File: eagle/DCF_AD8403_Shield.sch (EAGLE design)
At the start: 21 parts, among them IC1 TL072P, IC2 AD8403-100, J1 DCIN

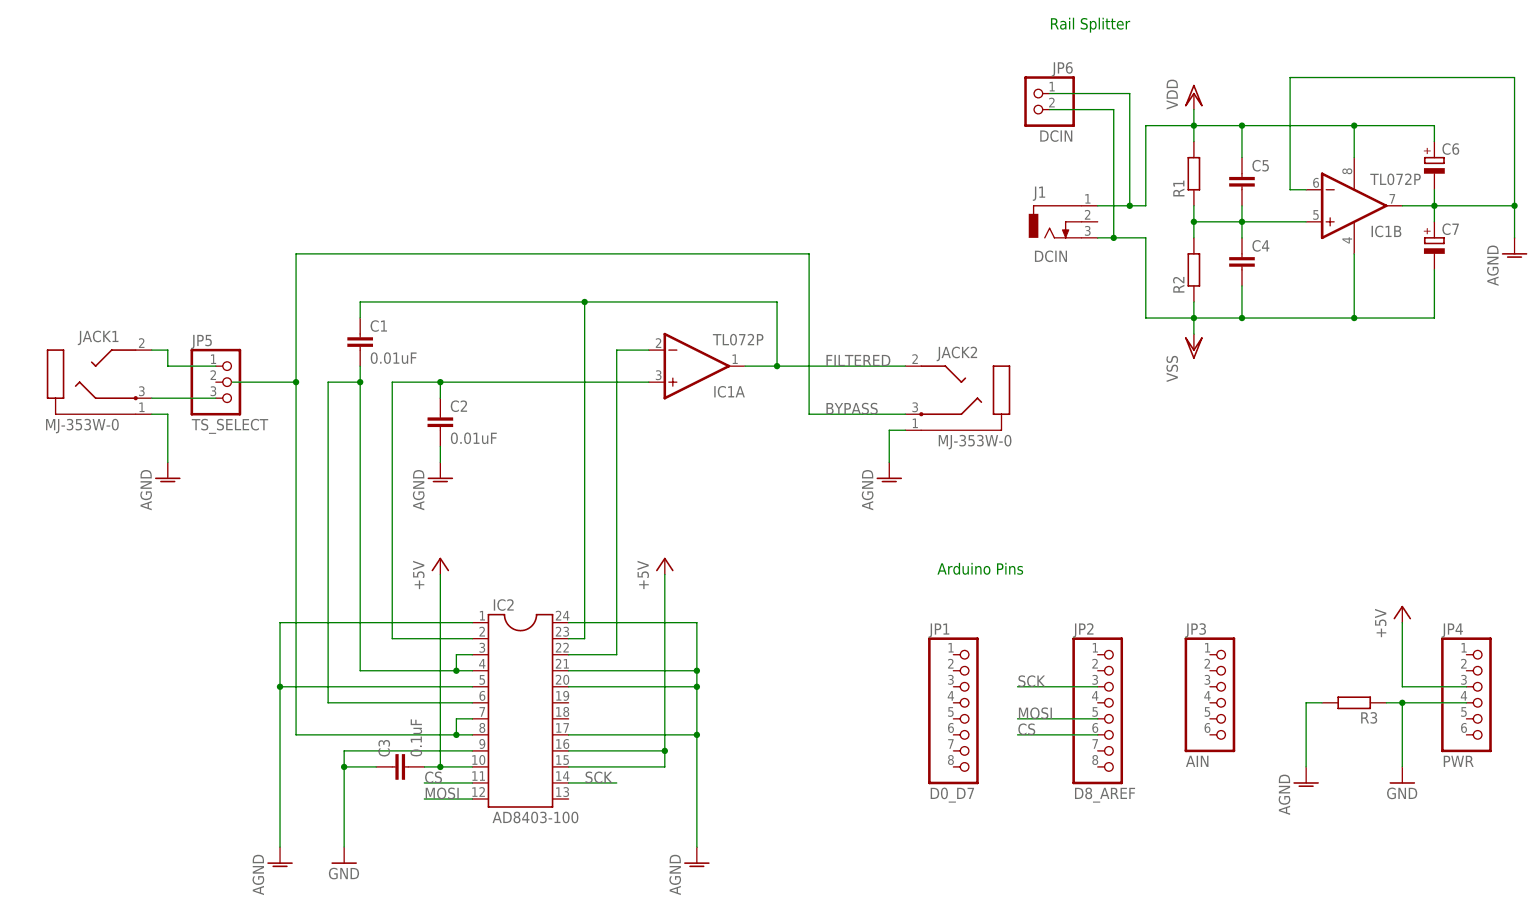
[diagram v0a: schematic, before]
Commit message: 基板図仮配線
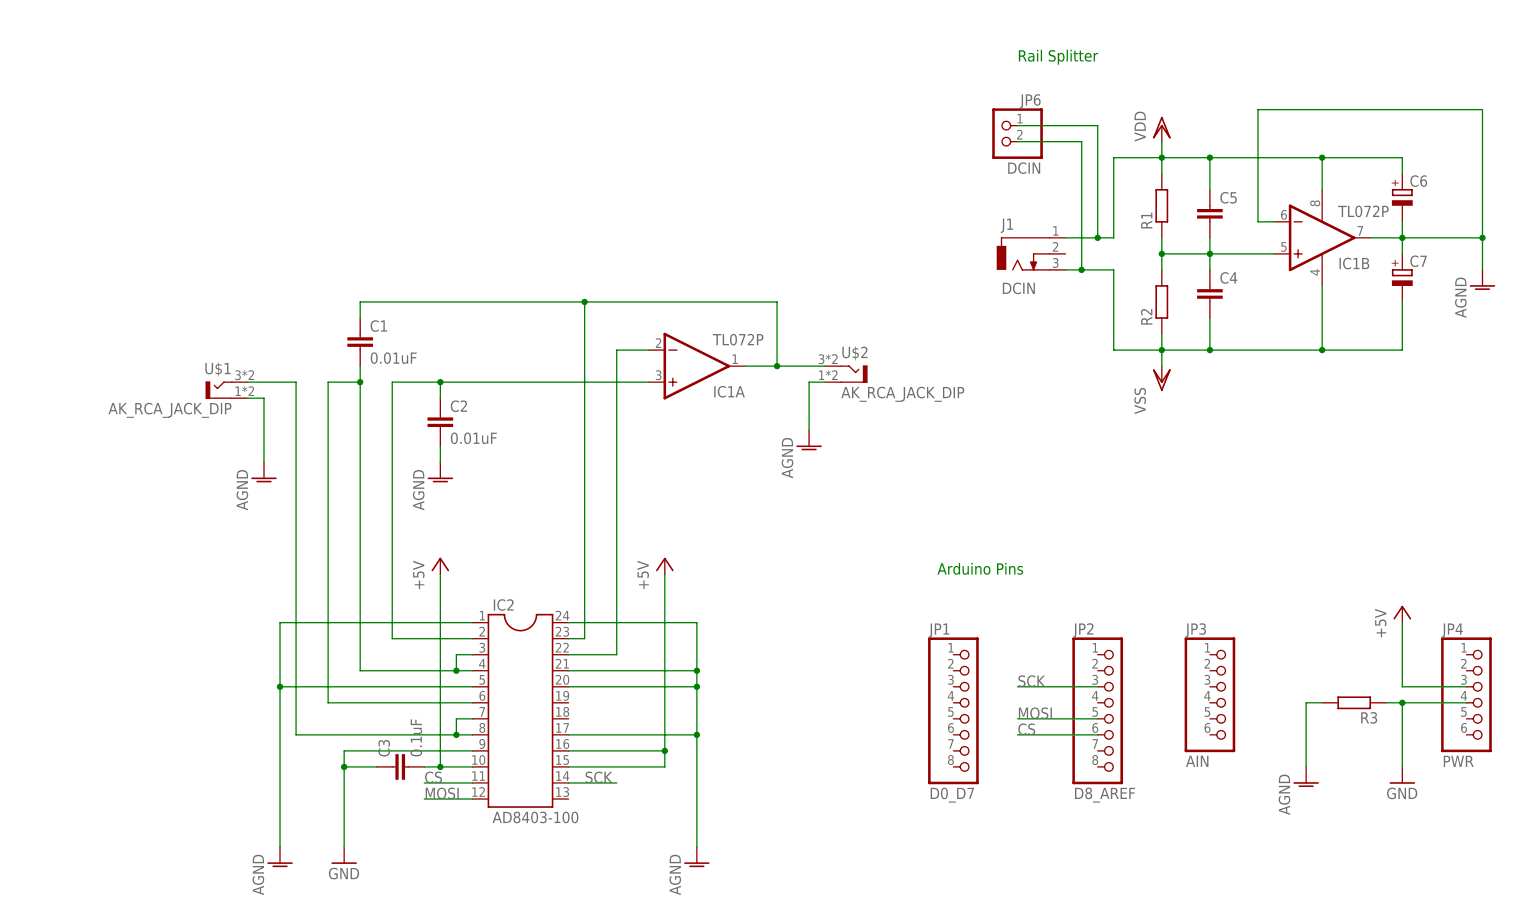
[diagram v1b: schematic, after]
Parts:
- removed JACK1, JACK2: MJ-353W-0, mylib2:MJ-353W-0
- removed JP5: TS_SELECT, pinhead:PINHD-1X3
- added U$1, U$2: AK_RCA_JACK_DIP, mylib2:AK_RCA_JACK_DIP
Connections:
- removed net N$2: JACK1.2, JP5.1
- removed net N$4: JACK1.3, JP5.3
- net AGND: now also U$1.S, U$2.S; no longer JACK1.1, JACK2.1
- net BYPASS: now also U$1.T; no longer JACK2.3
- net FILTERED: now also U$2.T; no longer JACK2.2
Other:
- moved on the sheet: C4, C5, C6, C7, IC1B, J1, JP6, R1, R2
